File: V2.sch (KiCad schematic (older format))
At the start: 72 parts, among them J1 Input voltage, J20 Boot0, J21 Bed Temp, J22 Boot1, J26 USB_A, J27 LCD, J3 Bed Heater, J32 USB_B, J6 Head2, J7 Head1, M3 Motor Z2, M4 Motor Z1, M5 Motor Y, M6 Motor X, Q1 STN4NF20L, Q2 STN4NF20L, Q3 04N03LA, Q4 04N03LA, Q5 04N03LA, Q6 04N03LA, SW1 Bed Level nozle, SW10 Button DOWN, SW11 Button UP, SW12 Bed Level, SW2 Boundary X, SW3 Boundary Y, SW4 Boundary Z1, SW5 Boundary Z2, SW6 Boundary E1, SW7 Boundary E2, SW8 Button BACK, SW9 Button OK, U1 LM2596S-5, U2 R-783.3-1.0, U3 STM32F105VCT6, U4 CP2104, Y1 hc49s

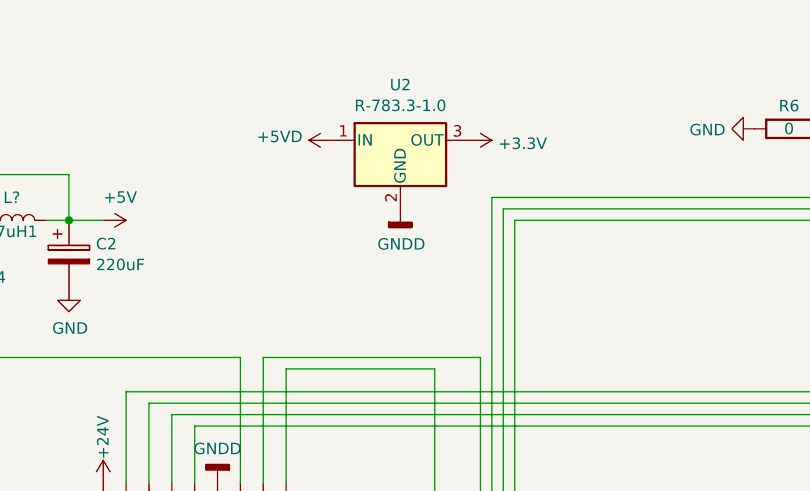
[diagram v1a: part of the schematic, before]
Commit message: переразвёл заново
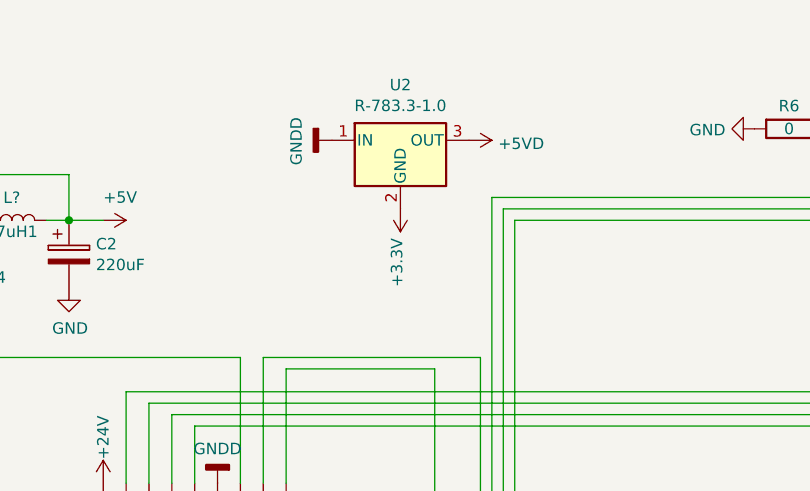
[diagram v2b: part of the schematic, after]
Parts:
- 47uH1: footprint Inductor_SMD:L_1206_3216Metric -> Inductor_THT:L_Radial_D12.0mm_P6.00mm_MuRATA_1900R
- C1: footprint Capacitor_SMD:CP_Elec_10x10.5 -> Capacitor_THT:CP_Radial_D10.0mm_P5.00mm
- C2: footprint Capacitor_SMD:CP_Elec_10x10.5 -> Capacitor_THT:CP_Radial_D10.0mm_P7.50mm
- D1: footprint Diode_SMD:D_2512_6332Metric_Castellated -> Diode_SMD:SS14
- D2: footprint w_smd_diode:do214ac -> w_smd_diode:do214ab
- J1, J3: footprint TerminalBlock_4Ucon:TerminalBlock_4Ucon_1x02_P3.50mm_Horizontal -> TerminalBlock_RND:TerminalBlock_RND_205-00045_1x02_P5.00mm_Horizontal
- Q1, Q2: footprint Package_TO_SOT_SMD:SOT-223-3_TabPin2 -> Package_TO_SOT_SMD:TO-252-2
- Q3, Q4, Q5, Q6: footprint Package_TO_SOT_SMD:TO-252-3_TabPin2 -> Package_TO_SOT_SMD:TO-252-2
- U2: footprint Package_TO_SOT_SMD:TO-252-3_TabPin2 -> Package_TO_SOT_SMD:SOT-223-3_TabPin2
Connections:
- net +3V3: now also U2.2 (GND); no longer U2.3 (OUT)
- net +5VD: now also U2.3 (OUT); no longer U2.1 (IN)
- net GNDD: now also U2.1 (IN); no longer U2.2 (GND)
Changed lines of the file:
@@
 L V2-rescue:GNDD-power #PWR0101
 U 1 1 5C43815D
-P 4450 1400
-F 0 "#PWR0101" H 4450 1150 50  0001 C CNN
-F 1 "GNDD" H 4454 1245 50  0000 C CNN
-F 2 "" H 4450 1400 50  0001 C CNN
-F 3 "" H 4450 1400 50  0001 C CNN
-	1    4450 1400
-	1    0    0    -1
+P 4150 1100
+F 0 "#PWR0101" H 4150 850 50  0001 C CNN
+F 1 "GNDD" H 4154 945 50  0000 C CNN
+F 2 "" H 4150 1100 50  0001 C CNN
+F 3 "" H 4150 1100 50  0001 C CNN
+	1    4150 1100
+	0    1    1    0
 $EndComp
 $Comp
@@
 F 0 "D1" V 2500 1650 50  0000 L CNN
 F 1 "SS54" V 2600 1650 50  0000 L CNN
-F 2 "Diode_SMD:D_2512_6332Metric_Castellated" H 2500 1425 50  0001 C CNN
+F 2 "Diode_SMD:SS14" H 2500 1425 50  0001 C CNN
 F 3 "http://www.vishay.com/docs/88526/1n5820.pdf" H 2500 1600 50  0001 C CNN
 	1    2500 1600
@@
 F 0 "47uH1" V 2700 1450 50  0000 C CNN
 F 1 "L?" V 2849 1450 50  0000 C CNN
-F 2 "Inductor_SMD:L_1206_3216Metric" H 2750 1450 50  0001 C CNN
+F 2 "Inductor_THT:L_Radial_D12.0mm_P6.00mm_MuRATA_1900R" H 2750 1450 50  0001 C CNN
 F 3 "" H 2750 1450 50  0001 C CNN
 	1    2750 1450
@@
 F 0 "C1" H 1132 954 50  0000 R CNN
 F 1 "680uF" H 1132 1045 50  0000 R CNN
-F 2 "Capacitor_SMD:CP_Elec_10x10.5" H 1288 850 50  0001 C CNN
+F 2 "Capacitor_THT:CP_Radial_D10.0mm_P5.00mm" H 1288 850 50  0001 C CNN
 F 3 "" H 1250 1000 50  0001 C CNN
 	1    1250 1000
@@
 F 0 "C2" H 3118 1646 50  0000 L CNN
 F 1 "220uF" H 3118 1555 50  0000 L CNN
-F 2 "Capacitor_SMD:CP_Elec_10x10.5" H 3038 1450 50  0001 C CNN
+F 2 "Capacitor_THT:CP_Radial_D10.0mm_P7.50mm" H 3038 1450 50  0001 C CNN
 F 3 "" H 3000 1600 50  0001 C CNN
 	1    3000 1600
@@
 L V2-rescue:+5VD-power #PWR0111
 U 1 1 5C44D470
-P 4150 1100
-F 0 "#PWR0111" H 4150 950 50  0001 C CNN
-F 1 "+5VD" V 4165 1228 50  0000 L CNN
-F 2 "" H 4150 1100 50  0001 C CNN
-F 3 "" H 4150 1100 50  0001 C CNN
-	1    4150 1100
-	0    -1   -1   0
+P 4750 1100
+F 0 "#PWR0111" H 4750 950 50  0001 C CNN
+F 1 "+5VD" V 4765 1228 50  0000 L CNN
+F 2 "" H 4750 1100 50  0001 C CNN
+F 3 "" H 4750 1100 50  0001 C CNN
+	1    4750 1100
+	0    1    1    0
 $EndComp
 $Comp
@@
 F 0 "D2" H 7400 834 50  0000 C CNN
 F 1 "1n5819" H 7400 925 50  0000 C CNN
-F 2 "w_smd_diode:do214ac" H 7400 1050 50  0001 C CNN
+F 2 "w_smd_diode:do214ab" H 7400 1050 50  0001 C CNN
 F 3 "" H 7400 1050 50  0001 C CNN
 	1    7400 1050
@@
 F 0 "U2" H 4450 1342 50  0000 C CNN
 F 1 "R-783.3-1.0" H 4450 1251 50  0000 C CNN
-F 2 "Package_TO_SOT_SMD:TO-252-3_TabPin2" H 4500 850 50  0001 L CIN
+F 2 "Package_TO_SOT_SMD:SOT-223-3_TabPin2" H 4500 850 50  0001 L CIN
 F 3 "https://www.recom-power.com/pdf/Innoline/R-78xx-1.0.pdf" H 4450 1100 50  0001 C CNN
 	1    4450 1100
@@
 L V2-rescue:+3.3V-power #PWR0118
 U 1 1 5C45FD0D
-P 4750 1100
-F 0 "#PWR0118" H 4750 950 50  0001 C CNN
-F 1 "+3.3V" V 4765 1228 50  0000 L CNN
-F 2 "" H 4750 1100 50  0001 C CNN
-F 3 "" H 4750 1100 50  0001 C CNN
-	1    4750 1100
-	0    1    1    0
+P 4450 1400
+F 0 "#PWR0118" H 4450 1250 50  0001 C CNN
+F 1 "+3.3V" V 4465 1528 50  0000 L CNN
+F 2 "" H 4450 1400 50  0001 C CNN
+F 3 "" H 4450 1400 50  0001 C CNN
+	1    4450 1400
+	-1   0    0    1
 $EndComp
 $Comp
@@
 F 0 "Q1" H 1006 4796 50  0000 L CNN
 F 1 "STN4NF20L" H 1006 4705 50  0000 L CNN
-F 2 "Package_TO_SOT_SMD:SOT-223-3_TabPin2" H 1000 4675 50  0001 L CIN
+F 2 "Package_TO_SOT_SMD:TO-252-2" H 1000 4675 50  0001 L CIN
 F 3 "https://www.infineon.com/dgdl/Infineon-BSP129-DS-v01_42-en.pdf?fileId=db3a30433c1a8752013c1fc296d2395f" H 800 4750 50  0001 L CNN
 	1    800  4750
@@
 F 0 "Q2" H 1906 4796 50  0000 L CNN
 F 1 "STN4NF20L" H 1906 4705 50  0000 L CNN
-F 2 "Package_TO_SOT_SMD:SOT-223-3_TabPin2" H 1900 4675 50  0001 L CIN
+F 2 "Package_TO_SOT_SMD:TO-252-2" H 1900 4675 50  0001 L CIN
 F 3 "https://www.infineon.com/dgdl/Infineon-BSP129-DS-v01_42-en.pdf?fileId=db3a30433c1a8752013c1fc296d2395f" H 1700 4750 50  0001 L CNN
 	1    1700 4750
@@
 F 0 "J3" V 2710 4241 50  0000 L CNN
 F 1 "Bed Heater" V 2550 3950 50  0000 L CNN
-F 2 "TerminalBlock_4Ucon:TerminalBlock_4Ucon_1x02_P3.50mm_Horizontal" H 2650 4200 50  0001 C CNN
+F 2 "TerminalBlock_RND:TerminalBlock_RND_205-00045_1x02_P5.00mm_Horizontal" H 2650 4200 50  0001 C CNN
 F 3 "~" H 2650 4200 50  0001 C CNN
 	1    2650 4200
@@
 F 0 "Q4" H 3550 4800 50  0000 L CNN
 F 1 "04N03LA" H 3550 4700 50  0000 L CNN
-F 2 "Package_TO_SOT_SMD:TO-252-3_TabPin2" H 3550 4675 50  0001 L CIN
+F 2 "Package_TO_SOT_SMD:TO-252-2" H 3550 4675 50  0001 L CIN
 F 3 "https://www.fairchildsemi.com/datasheets/BS/BSS138.pdf" H 3350 4750 50  0001 L CNN
 	1    3350 4750
@@
 F 0 "Q3" H 2750 4800 50  0000 L CNN
 F 1 "04N03LA" H 2750 4700 50  0000 L CNN
-F 2 "Package_TO_SOT_SMD:TO-252-3_TabPin2" H 2750 4675 50  0001 L CIN
+F 2 "Package_TO_SOT_SMD:TO-252-2" H 2750 4675 50  0001 L CIN
 F 3 "https://www.fairchildsemi.com/datasheets/BS/BSS138.pdf" H 2550 4750 50  0001 L CNN
 	1    2550 4750
@@
 F 0 "Q5" H 4400 4800 50  0000 L CNN
 F 1 "04N03LA" H 4400 4700 50  0000 L CNN
-F 2 "Package_TO_SOT_SMD:TO-252-3_TabPin2" H 4400 4675 50  0001 L CIN
+F 2 "Package_TO_SOT_SMD:TO-252-2" H 4400 4675 50  0001 L CIN
 F 3 "https://www.fairchildsemi.com/datasheets/BS/BSS138.pdf" H 4200 4750 50  0001 L CNN
 	1    4200 4750
@@
 F 0 "Q6" H 20750 10550 50  0000 L CNN
 F 1 "04N03LA" H 20750 10450 50  0000 L CNN
-F 2 "Package_TO_SOT_SMD:TO-252-3_TabPin2" H 20750 10425 50  0001 L CIN
+F 2 "Package_TO_SOT_SMD:TO-252-2" H 20750 10425 50  0001 L CIN
 F 3 "https://www.fairchildsemi.com/datasheets/BS/BSS138.pdf" H 20550 10500 50  0001 L CNN
 	1    20550 10500
@@
 F 0 "J1" V 10973 1180 50  0000 L CNN
 F 1 "Input voltage" V 11064 1180 50  0000 L CNN
-F 2 "TerminalBlock_4Ucon:TerminalBlock_4Ucon_1x02_P3.50mm_Horizontal" H 11100 1100 50  0001 C CNN
+F 2 "TerminalBlock_RND:TerminalBlock_RND_205-00045_1x02_P5.00mm_Horizontal" H 11100 1100 50  0001 C CNN
 F 3 "~" H 11100 1100 50  0001 C CNN
 	1    11100 1100
